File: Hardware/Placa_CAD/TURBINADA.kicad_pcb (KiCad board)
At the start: 4 copper layers, 110 x 102 mm, 49 parts, among them J1 TURBINA, J2 RESISTENCIAS, J3 BATERIA, J4 ICSP, Q1 IXTP44P15T, Q2 IXTP36P15P, Q3 FQN1N50C, Q4 FQN1N50C, U1 PIC16F18324-xSL, U2 ADP2302ARDZ-5.0

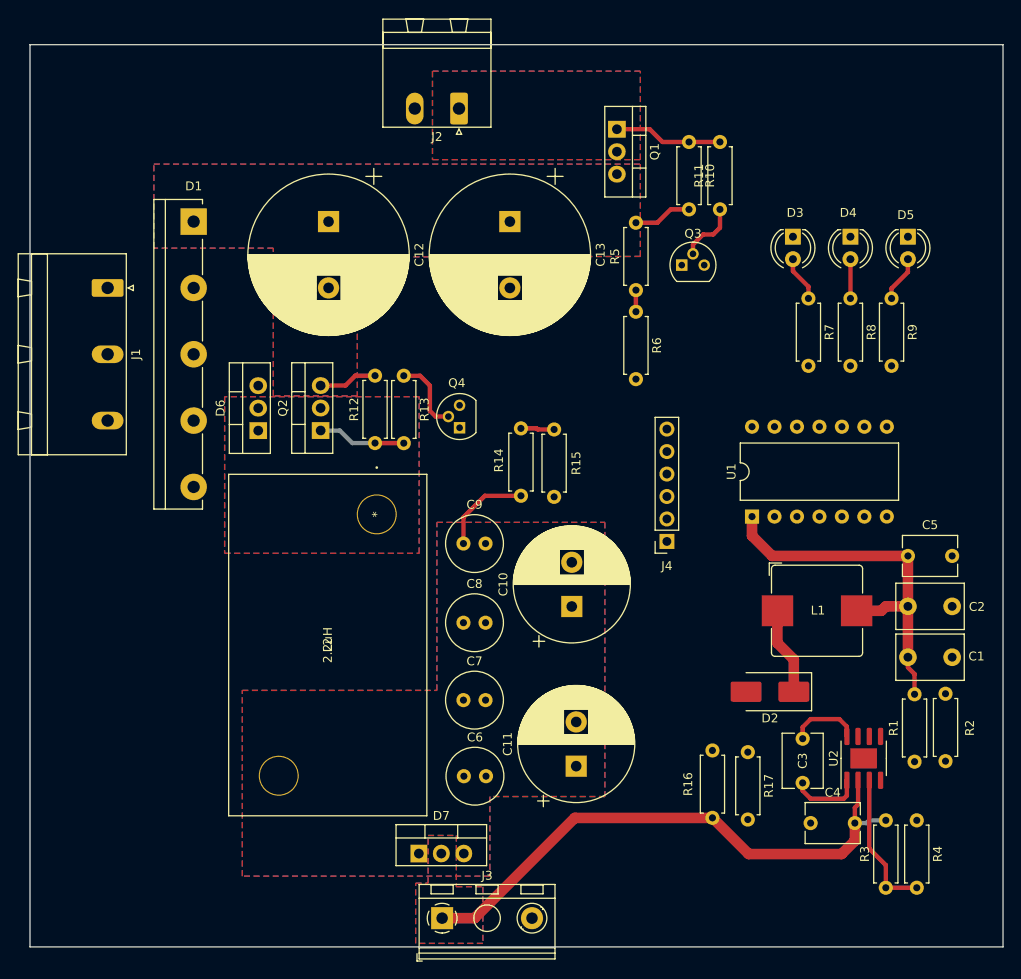
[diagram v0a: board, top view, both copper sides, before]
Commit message: Finished board layout
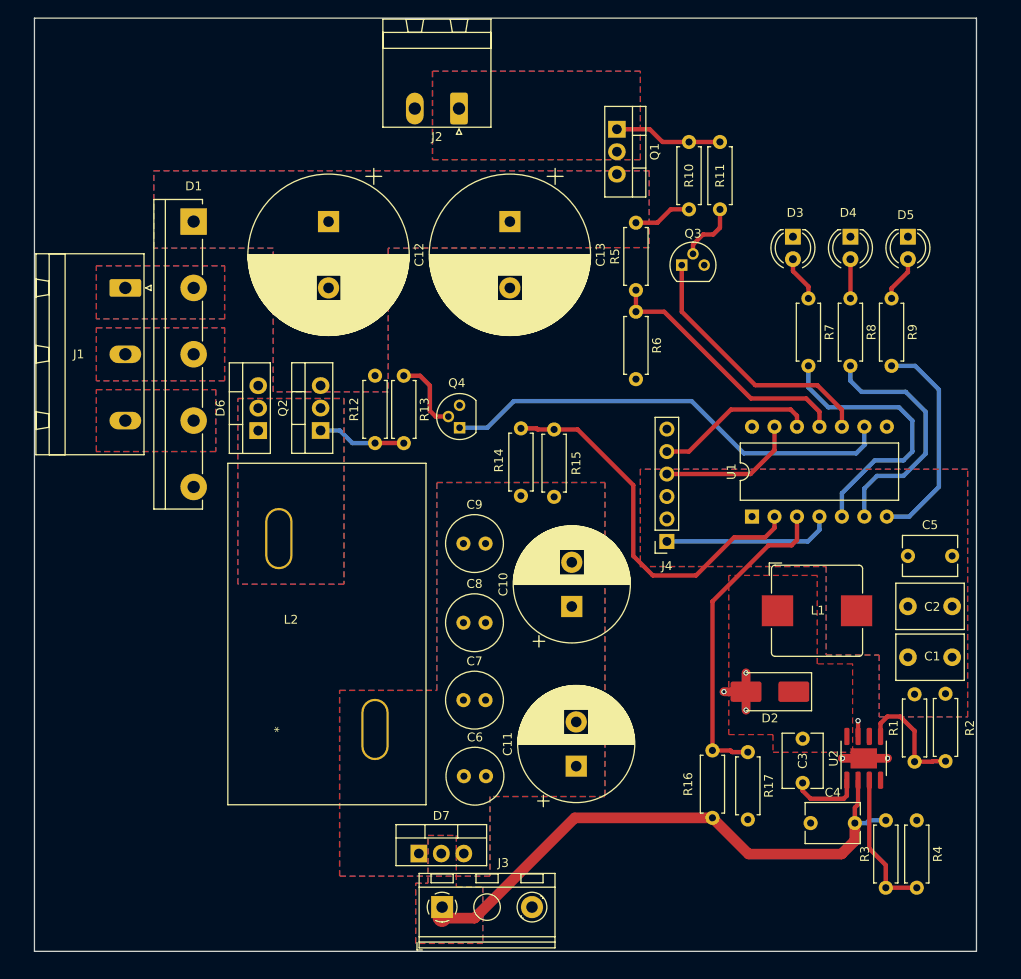
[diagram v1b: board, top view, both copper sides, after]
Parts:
- L2: footprint footprints:IHXL1500VZEB1R5M51 -> footprints:IHXL1500VZEB2R2M51
- R1: value 10K -> 52.3K
- R2: value 5K -> 10K
- moved L2 26.7 mm to (174.1, 115.4), turned to 90 degrees
- moved J1 2.00 mm to (156.8, 65.5)
- moved J3 1.25 mm to (192.6, 135.5)
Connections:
- L2 pad 1: Net-(D6-K) -> Net-(C10-Pad1)
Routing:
- net Net-(Q4-G): track 0.00 -> 52.0 mm
- net +5V: track 42.7 -> 0.00 mm
- net OUT_VOLTAGE: track 3.80 -> 43.7 mm
- net BAT_VOLTAGE: track 0.00 -> 36.0 mm
- net Net-(U1-RC5): track 0.00 -> 31.8 mm
- net Net-(Q3-G): track 0.00 -> 29.9 mm
- net Net-(U1-RC4): track 0.00 -> 28.1 mm
- net Net-(U1-RA2): track 2.44 -> 29.6 mm
- net Net-(U1-RC3): track 0.00 -> 24.7 mm
- net Net-(J4-Pin_1): track 0.00 -> 19.3 mm
- net Net-(J4-Pin_5): track 0.00 -> 18.2 mm
- net Net-(D2-K): track 18.1 -> 0.00 mm
- net Net-(J4-Pin_4): track 0.00 -> 15.9 mm
- net GND: track 0.00 -> 13.6 mm, vias 0 -> 6
- net Net-(U2-FB): track 0.00 -> 13.3 mm
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- added copper zone on B.Cu, net +5V
- added copper zone on F.Cu, net +5V
- added copper zone on In1.Cu, net +5V
- added copper zone on In4.Cu, net +5V
- added copper zone on In1.Cu, net /VCC Turbina (0 ~ 115V)
- added copper zone on In4.Cu, net /VCC Turbina (0 ~ 115V)
- added copper zone on In2.Cu, net GND
- added copper zone on In3.Cu, net GND
- added copper zone on In1.Cu, net Net-(C10-Pad1)
- added copper zone on In4.Cu, net Net-(C10-Pad1)
- added copper zone on F.Cu, net Net-(D2-K)
- added copper zone on In1.Cu, net Net-(D6-K)
- added copper zone on In4.Cu, net Net-(D6-K)
- added copper zone on In1.Cu, net Net-(D7-K)
- added copper zone on In4.Cu, net Net-(D7-K)
- added copper zone on B.Cu, net Net-(J1-Pin_1)
- added copper zone on F.Cu, net Net-(J1-Pin_1)
- added copper zone on In1.Cu, net Net-(J1-Pin_1)
- added copper zone on In4.Cu, net Net-(J1-Pin_1)
- added copper zone on B.Cu, net Net-(J1-Pin_2)
- added copper zone on F.Cu, net Net-(J1-Pin_2)
- added copper zone on In1.Cu, net Net-(J1-Pin_2)
- added copper zone on In4.Cu, net Net-(J1-Pin_2)
- added copper zone on B.Cu, net Net-(J1-Pin_3)
- added copper zone on F.Cu, net Net-(J1-Pin_3)
- added copper zone on In1.Cu, net Net-(J1-Pin_3)
- added copper zone on In4.Cu, net Net-(J1-Pin_3)
- added copper zone on In1.Cu, net Net-(J2-Pin_1)
- added copper zone on In4.Cu, net Net-(J2-Pin_1)
- removed copper zone on In1.Cu, net GND
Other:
- board size 110 x 102 mm -> 106.5 x 105.5 mm
- copper layers 4 -> 6
